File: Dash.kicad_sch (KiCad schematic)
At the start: 152 parts, among them J10 Conn_01x04_Socket, J11 Conn_01x04_Socket, J12 Conn_01x06_Socket, J13 Conn_01x06_Socket, J14 Conn_01x06_Socket, J15 Conn_01x06_Socket, J2 Conn_01x06_Socket, J4 Conn_01x03_Socket, J5 Conn_01x04_Socket, J6 Conn_01x04_Socket, J7 Conn_01x04_Socket, J8 Conn_01x04_Socket, J9 Conn_01x04_Socket, Q1 NPN, Q10 NPN, Q11 NPN, Q12 NPN, Q13 NPN, Q14 NPN, Q15 NPN, Q16 NPN, Q17 NPN, Q18 NPN, Q19 PMOS, Q2 NPN, Q20 NMOS, Q21 NPN, Q3 NPN, Q4 NPN, Q5 NPN, Q6 NPN, Q7 NPN, Q8 NPN, Q9 NPN, SW1 SW_Push, U1 LM2678T-5.0, U10 L293D, U11 L293D, U12 L293D, U13 L293D, U14 L293D, U15 L293D, U16 SFH617A-1, U2 ADS1015IDGS, U4 24C02Cx-x-SN, U5 ESP32-S2-DevKitM, U6 24C02Cx-x-SN, U7 74HC595, U8 74HC595, U9 74HC595

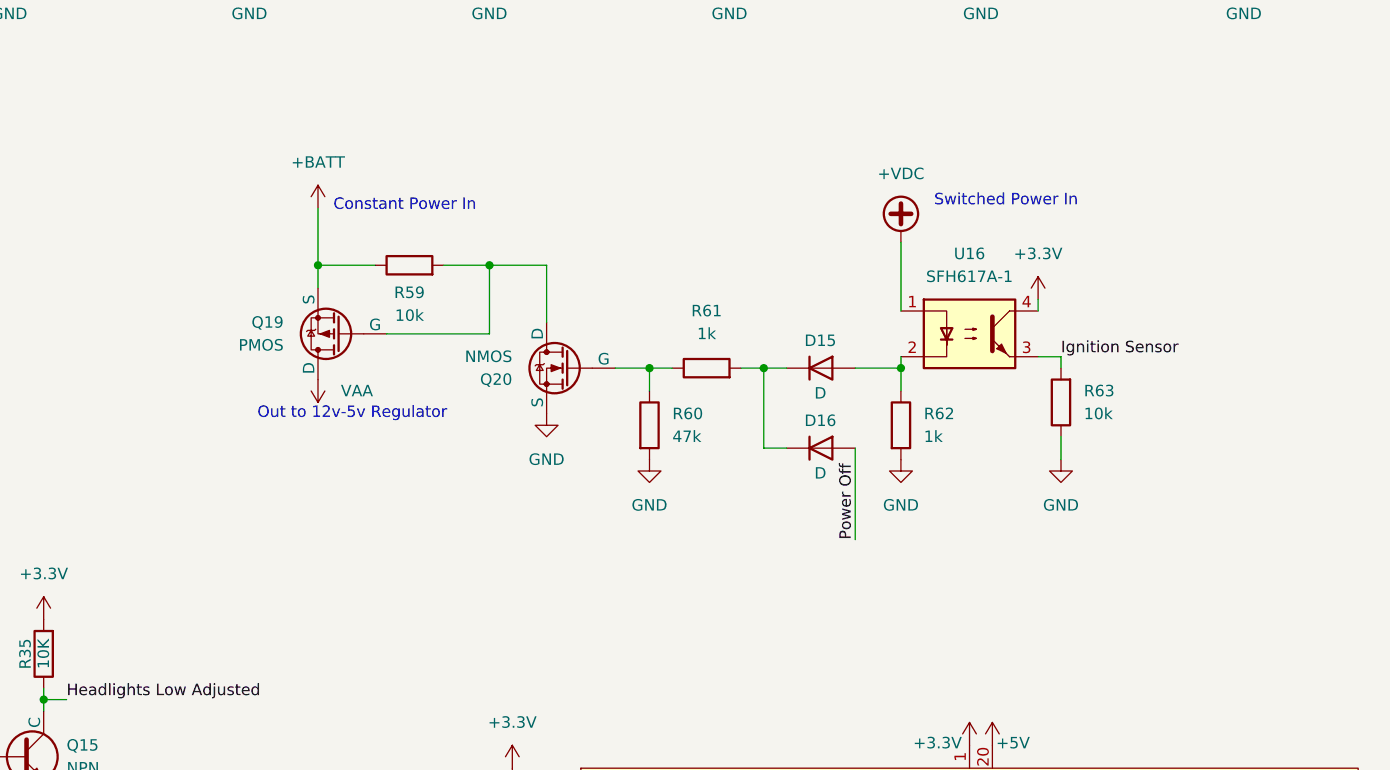
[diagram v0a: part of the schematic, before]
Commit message: Update Dash.kicad_sch
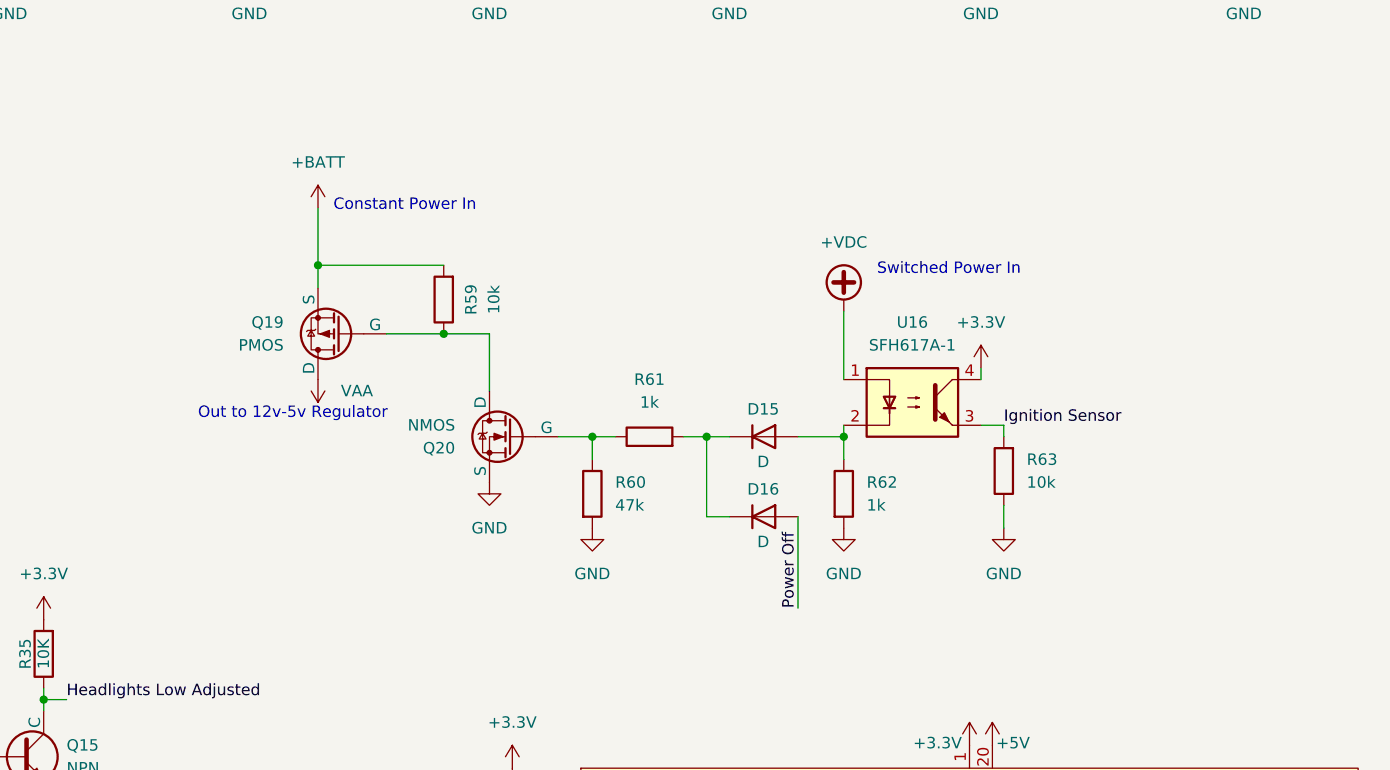
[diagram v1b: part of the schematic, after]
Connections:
- net +BATT: now also R59.2; no longer R59.1
- net at Q19.2 (G), Q20.1 (D): now also R59.1; no longer R59.2
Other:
- moved on the sheet: D15, D16, Q20, R59, R60, R61, R62, R63, U16
